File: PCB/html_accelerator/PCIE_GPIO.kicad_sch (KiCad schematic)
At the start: 1 part, among them U1 MCS9990

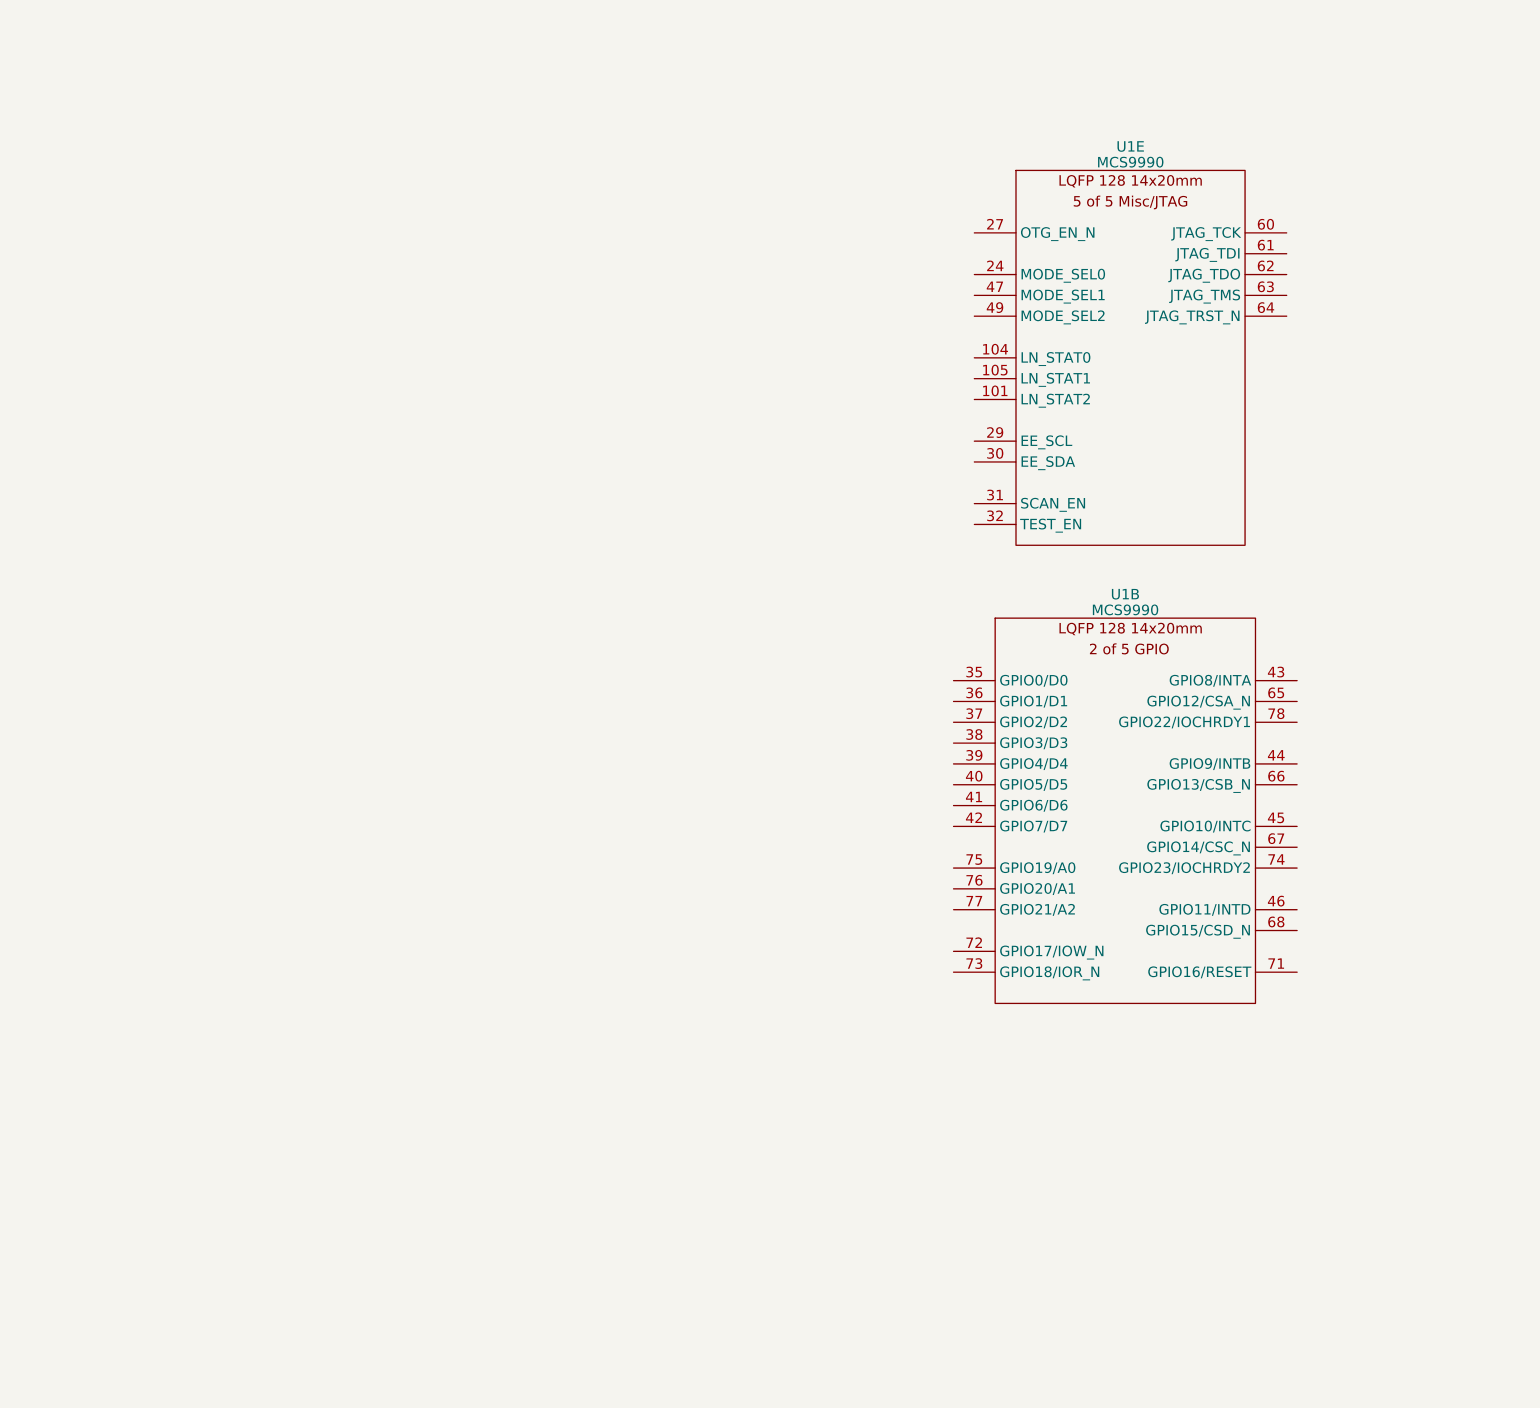
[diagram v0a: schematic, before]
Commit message: schematic updates
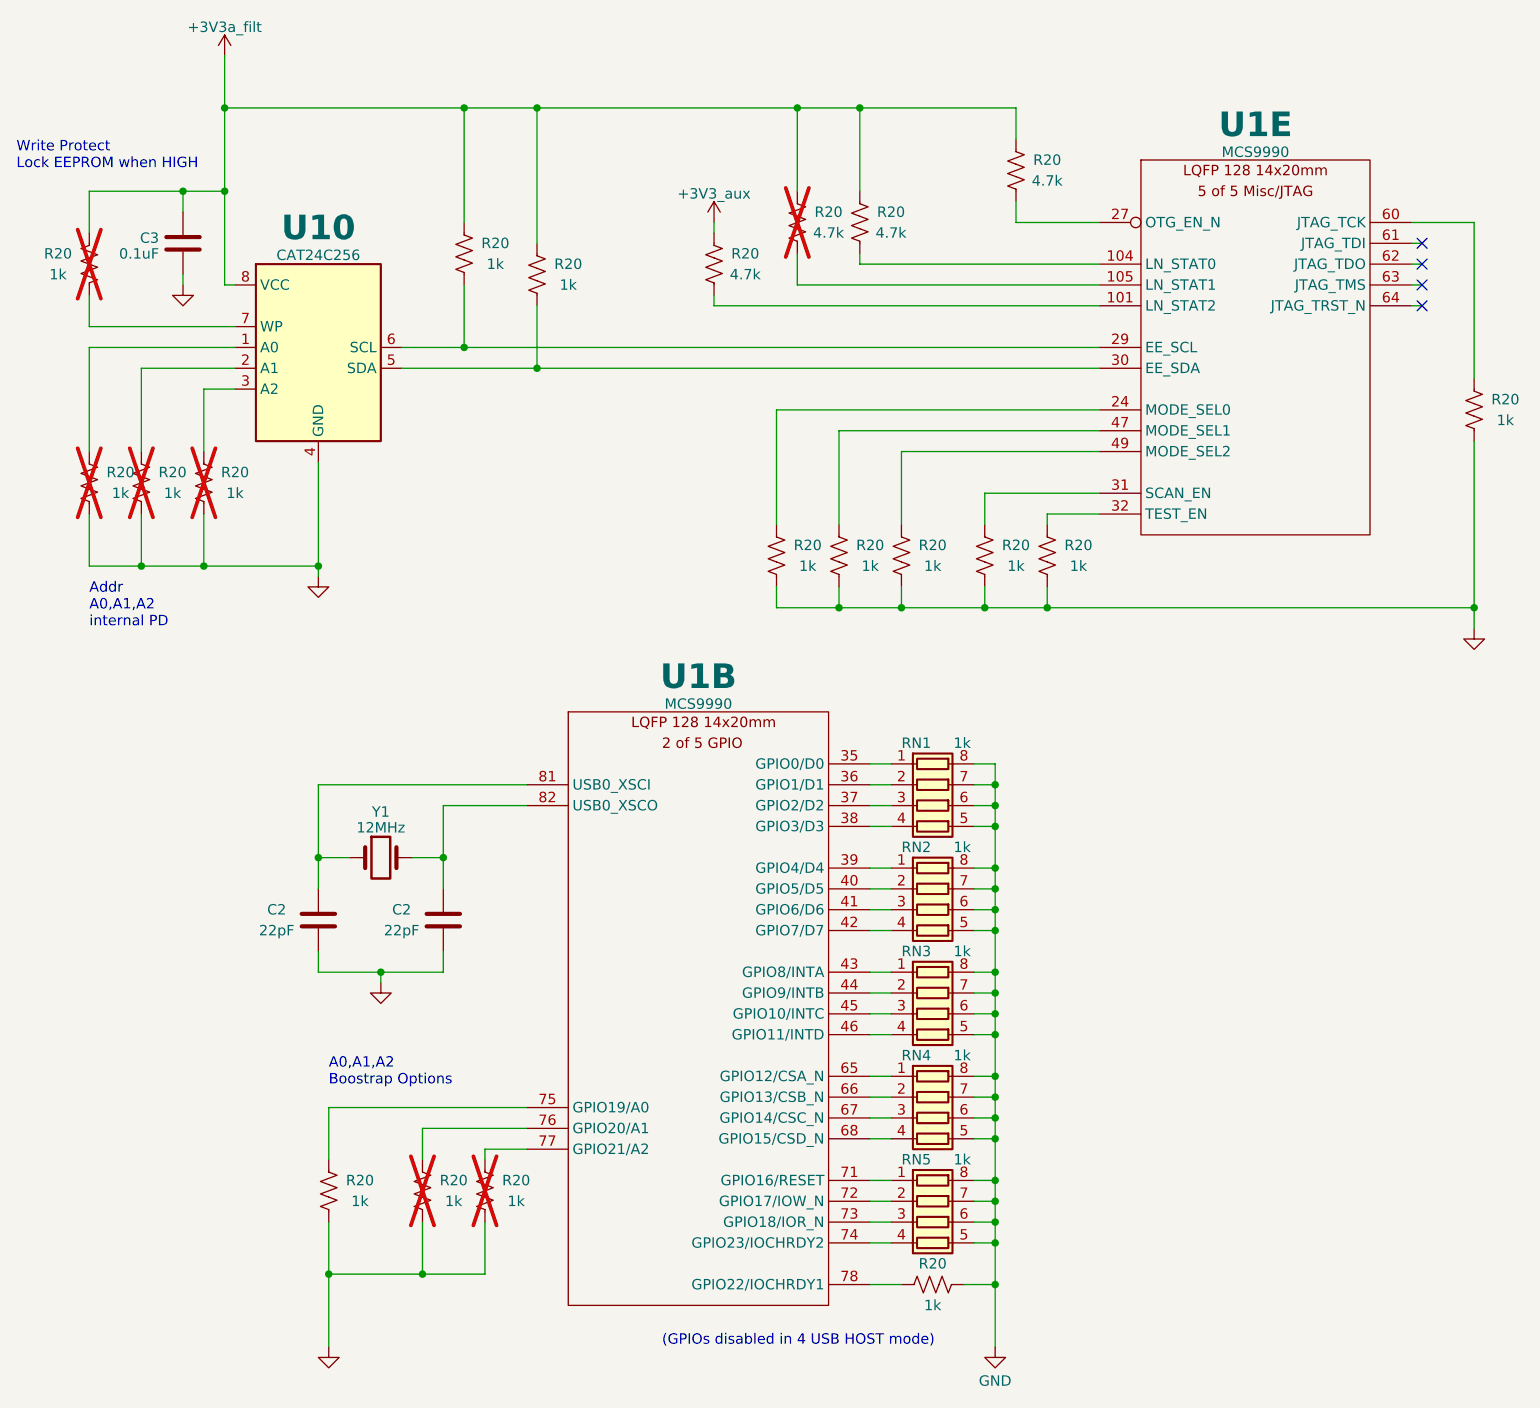
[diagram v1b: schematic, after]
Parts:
- added C2 (x2): 22pF, symbol Device:C
- added C3: 0.1uF, symbol Device:C
- added R20 (x4): 4.7k, symbol Device:R_US
- added R20 (x16): 1k, symbol Device:R_US
- added RN1, RN2, RN3, RN4, RN5: 1k, symbol Device:R_Pack04
- added U10: CAT24C256, symbol Memory_EEPROM:CAT24C256
- added Y1: 12MHz, symbol Device:Crystal
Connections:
- net at U1.35 (GPIO0/D0): now also RN1.1 (R1.1)
- net at U1.36 (GPIO1/D1): now also RN1.2 (R2.1)
- net at U1.37 (GPIO2/D2): now also RN1.3 (R3.1)
- net at U1.38 (GPIO3/D3): now also RN1.4 (R4.1)
- net at U1.39 (GPIO4/D4): now also RN2.1 (R1.1)
- net at U1.40 (GPIO5/D5): now also RN2.2 (R2.1)
- net at U1.41 (GPIO6/D6): now also RN2.3 (R3.1)
- net at U1.42 (GPIO7/D7): now also RN2.4 (R4.1)
- net at U1.43 (GPIO8/INTA): now also RN3.1 (R1.1)
- net at U1.44 (GPIO9/INTB): now also RN3.2 (R2.1)
- net at U1.45 (GPIO10/INTC): now also RN3.3 (R3.1)
- net at U1.46 (GPIO11/INTD): now also RN3.4 (R4.1)
- net at U1.65 (GPIO12/CSA_N): now also RN4.1 (R1.1)
- net at U1.66 (GPIO13/CSB_N): now also RN4.2 (R2.1)
- net at U1.67 (GPIO14/CSC_N): now also RN4.3 (R3.1)
- net at U1.68 (GPIO15/CSD_N): now also RN4.4 (R4.1)
- net at U1.71 (GPIO16/RESET): now also RN5.1 (R1.1)
- net at U1.72 (GPIO17/IOW_N): now also RN5.2 (R2.1)
- net at U1.73 (GPIO18/IOR_N): now also RN5.3 (R3.1)
- net at U1.74 (GPIO23/IOCHRDY2): now also RN5.4 (R4.1)
- net at U1.75 (GPIO19/A0): now also R20.1
- net at U1.76 (GPIO20/A1): now also R20.1
- net at U1.77 (GPIO21/A2): now also R20.1
- net at U1.78 (GPIO22/IOCHRDY1): now also R20.2
- net at U1.101 (LN_STAT2): now also R20.2
- net at U1.104 (LN_STAT0): now also R20.2
- net at U1.105 (LN_STAT1): now also R20.2
- net at U1.24 (MODE_SEL0): now also R20.1
- net at U1.27 (OTG_EN_N): now also R20.2
- net at U1.29 (EE_SCL): now also R20.2, U10.6 (SCL)
- net at U1.30 (EE_SDA): now also R20.2, U10.5 (SDA)
- net at U1.31 (SCAN_EN): now also R20.1
- net at U1.32 (TEST_EN): now also R20.1
- net at U1.47 (MODE_SEL1): now also R20.1
- net at U1.49 (MODE_SEL2): now also R20.1
- net at U1.60 (JTAG_TCK): now also R20.1
- new net: C2.1, U1.81 (USB0_XSCI), Y1.1
- new net: C2.1, U1.82 (USB0_XSCO), Y1.2
- new net: R20.1, U10.3 (A2)
- new net: R20.1, U10.1 (A0)
- new net: R20.1, U10.2 (A1)
- new net: R20.2, U10.7 (WP)
- new net +3V3: C3.2, R20.1, R20.1, R20.1, R20.1, R20.1, R20.1, R20.1, U10.8 (VCC)
- new net GND: C2.2, C2.2, C3.1, R20.1, R20.2, R20.2, R20.2, R20.2, R20.2, R20.2, R20.2, R20.2, R20.2, R20.2, R20.2, R20.2, RN1.5 (R4.2), RN1.6 (R3.2), RN1.7 (R2.2), RN1.8 (R1.2), RN2.5 (R4.2), RN2.6 (R3.2), RN2.7 (R2.2), RN2.8 (R1.2), RN3.5 (R4.2), RN3.6 (R3.2), RN3.7 (R2.2), RN3.8 (R1.2), RN4.5 (R4.2), RN4.6 (R3.2), RN4.7 (R2.2), RN4.8 (R1.2), RN5.5 (R4.2), RN5.6 (R3.2), RN5.7 (R2.2), RN5.8 (R1.2), U10.4 (GND)
- no-connect marks 0 -> 4
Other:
- note added: "(GPIOs disabled in 4 USB HOST mode)"
- note added: "A0,A1,A2 Boostrap Options"
- note added: "Addr A0,A1,A2 internal PD"
- note added: "Write Protect Lock EEPROM when HIGH"
- title: (none) -> EEPROM, CFG, GPIO
